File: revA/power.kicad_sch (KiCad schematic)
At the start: 58 parts, among them J9 Conn_02x02_Top_Bottom, Q1 MMBT4401WT1G, Q3 BSZ180, Q3 MMDT2222A, Q4 IRLML2803, Q6 MMDT2222A, Q9 MMDT2222A, U25 AP2161W, U3 MCP1700T-50, U4 MCP1700T-33, U5 MCP1700T-33, U6 ATL431BQ

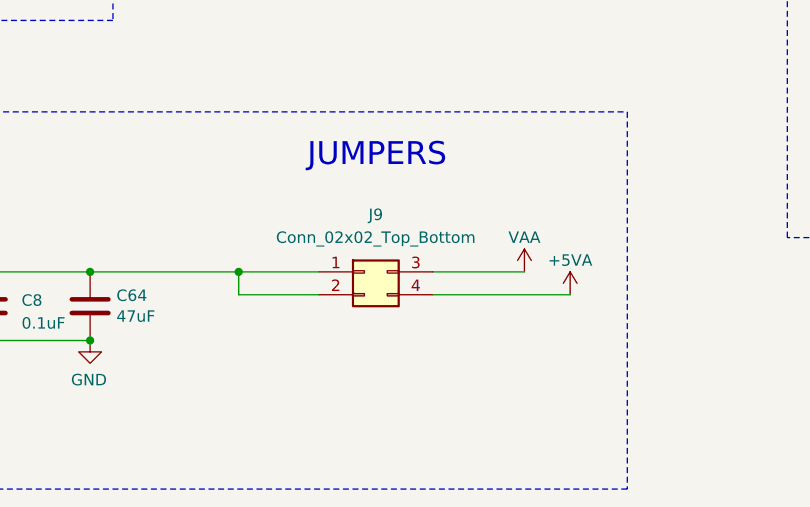
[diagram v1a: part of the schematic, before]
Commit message: placement
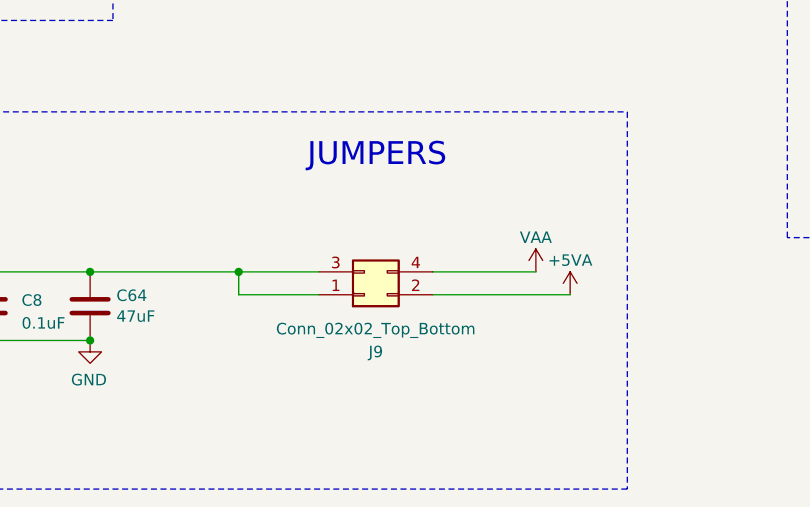
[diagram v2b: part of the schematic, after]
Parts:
- J9: symbol Connector_Generic:Conn_02x02_Top_Bottom -> Connector_Generic:Conn_02x02_Odd_Even
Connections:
- net +5VA: now also J9.2 (Pin_2); no longer J9.4 (Pin_4)
- net VAA: now also J9.4 (Pin_4); no longer J9.3 (Pin_3)
- net at C64.1, C8.1, J9.1 (Pin_1)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: now also J9.3 (Pin_3); no longer J9.2 (Pin_2)
- removed net +3V3: C13.1, C16.1, C17.1, R8.2, R87.1, R9.1, TP3.1, TP3.1, TP3.1, U4.3 (VO), U5.3 (VO), U6.2 (K)
- new net +1V65A: C17.1, R8.2, R9.1, TP3.1, U6.2 (K)
- new net +3V3A: C16.1, TP3.1, U5.3 (VO)
- new net +3V3D: C13.1, R87.1, TP3.1, U4.3 (VO)
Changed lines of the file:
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@@
     (stroke (width 0) (type default))
   )
-  (wire (pts (xy 182.88 215.9) (xy 193.04 215.9))
+  (wire (pts (xy 182.88 218.44) (xy 198.12 218.44))
     (stroke (width 0) (type default))
   )
@@
     (stroke (width 0) (type default))
   )
-  (wire (pts (xy 161.29 215.9) (xy 170.18 215.9))
-    (stroke (width 0) (type default))
-  )
   (wire (pts (xy 80.01 161.29) (xy 87.63 161.29))
     (stroke (width 0) (type default))
@@
     (stroke (width 0) (type default))
   )
+  (wire (pts (xy 161.29 215.9) (xy 170.18 215.9))
+    (stroke (width 0) (type default))
+  )
   (wire (pts (xy 63.5 55.88) (xy 95.25 55.88))
     (stroke (width 0) (type default))
@@
     (stroke (width 0) (type default))
   )
-  (wire (pts (xy 182.88 218.44) (xy 198.12 218.44))
+  (wire (pts (xy 182.88 215.9) (xy 194.31 215.9))
     (stroke (width 0) (type default))
   )
@@
       (effects (font (size 1.27 1.27)) hide)
     )
+    (property "Manufacturer" "" (at 351.79 170.18 0)
+      (effects (font (size 1.27 1.27)) hide)
+    )
+    (property "Mfr. Part No" "" (at 351.79 170.18 0)
+      (effects (font (size 1.27 1.27)) hide)
+    )
+    (property "Description" "" (at 351.79 170.18 0)
+      (effects (font (size 1.27 1.27)) hide)
+    )
     (pin "1")
     (instances
@@
       (effects (font (size 1.27 1.27)) hide)
     )
+    (property "Manufacturer" "" (at 309.88 175.26 0)
+      (effects (font (size 1.27 1.27)) hide)
+    )
+    (property "Mfr. Part No" "" (at 309.88 175.26 0)
+      (effects (font (size 1.27 1.27)) hide)
+    )
+    (property "Description" "" (at 309.88 175.26 0)
+      (effects (font (size 1.27 1.27)) hide)
+    )
     (pin "1")
     (instances
@@
     )
   )
-  (symbol (lib_id "Connector_Generic:Conn_02x02_Top_Bottom") (at 175.26 215.9 0) (unit 1)
+  (symbol (lib_id "Connector_Generic:Conn_02x02_Odd_Even") (at 175.26 218.44 0) (mirror x) (unit 1)
     (in_bom yes) (on_board yes) (dnp no)
-    (property "Reference" "J9" (at 176.53 209.55 0)
+    (property "Reference" "J9" (at 176.53 224.79 0)
       (effects (font (size 1.27 1.27)))
     )
-    (property "Value" "Conn_02x02_Top_Bottom" (at 176.53 212.09 0)
+    (property "Value" "Conn_02x02_Top_Bottom" (at 176.53 222.25 0)
       (effects (font (size 1.27 1.27)))
     )
-    (property "Footprint" "Connector_PinHeader_2.54mm:PinHeader_2x02_P2.54mm_Vertical_SMD" (at 175.26 215.9 0)
+    (property "Footprint" "Connector_PinHeader_2.54mm:PinHeader_2x02_P2.54mm_Vertical_SMD" (at 175.26 218.44 0)
+      (effects (font (size 1.27 1.27)) hide)
+    )
+    (property "Datasheet" "~" (at 175.26 218.44 0)
+      (effects (font (size 1.27 1.27)) hide)
+    )
+    (property "Manufacturer" "" (at 175.26 218.44 0)
       (effects (font (size 1.27 1.27)) hide)
     )
-    (property "Datasheet" "~" (at 175.26 215.9 0)
+    (property "Mfr. Part No" "" (at 175.26 218.44 0)
+      (effects (font (size 1.27 1.27)) hide)
+    )
+    (property "Description" "" (at 175.26 218.44 0)
       (effects (font (size 1.27 1.27)) hide)
     )
@@
       (effects (font (size 1.27 1.27)) hide)
     )
+    (property "Manufacturer" "" (at 309.88 160.02 0)
+      (effects (font (size 1.27 1.27)) hide)
+    )
+    (property "Mfr. Part No" "" (at 309.88 160.02 0)
+      (effects (font (size 1.27 1.27)) hide)
+    )
+    (property "Description" "" (at 309.88 160.02 0)
+      (effects (font (size 1.27 1.27)) hide)
+    )
     (pin "1")
     (instances
@@
       (effects (font (size 1.27 1.27)) hide)
     )
+    (property "Manufacturer" "" (at 281.94 184.15 0)
+      (effects (font (size 1.27 1.27)) hide)
+    )
+    (property "Mfr. Part No" "" (at 281.94 184.15 0)
+      (effects (font (size 1.27 1.27)) hide)
+    )
+    (property "Description" "" (at 281.94 184.15 0)
+      (effects (font (size 1.27 1.27)) hide)
+    )
     (pin "1")
     (instances
@@
       (effects (font (size 1.27 1.27)) hide)
     )
+    (property "Manufacturer" "" (at 271.78 45.72 0)
+      (effects (font (size 1.27 1.27)) hide)
+    )
+    (property "Mfr. Part No" "" (at 271.78 45.72 0)
+      (effects (font (size 1.27 1.27)) hide)
+    )
+    (property "Description" "" (at 271.78 45.72 0)
+      (effects (font (size 1.27 1.27)) hide)
+    )
     (pin "1")
     (instances
@@
       (effects (font (size 1.27 1.27)) hide)
     )
+    (property "Manufacturer" "" (at 309.88 182.88 0)
+      (effects (font (size 1.27 1.27)) hide)
+    )
+    (property "Mfr. Part No" "" (at 309.88 182.88 0)
+      (effects (font (size 1.27 1.27)) hide)
+    )
+    (property "Description" "" (at 309.88 182.88 0)
+      (effects (font (size 1.27 1.27)) hide)
+    )
     (pin "1")
     (instances
@@
       (effects (font (size 1.27 1.27)) hide)
     )
+    (property "Manufacturer" "" (at 271.78 137.16 0)
+      (effects (font (size 1.27 1.27)) hide)
+    )
+    (property "Mfr. Part No" "" (at 271.78 137.16 0)
+      (effects (font (size 1.27 1.27)) hide)
+    )
+    (property "Description" "" (at 271.78 137.16 0)
+      (effects (font (size 1.27 1.27)) hide)
+    )
     (pin "1")
     (instances
@@
     )
   )
-  (symbol (lib_id "power:VAA") (at 193.04 215.9 0) (unit 1)
+  (symbol (lib_id "power:VAA") (at 194.31 215.9 0) (unit 1)
     (in_bom yes) (on_board yes) (dnp no) (fields_autoplaced)
-    (property "Reference" "#PWR017" (at 193.04 219.71 0)
+    (property "Reference" "#PWR017" (at 194.31 219.71 0)
       (effects (font (size 1.27 1.27)) hide)
     )
-    (property "Value" "VAA" (at 193.04 212.09 0)
+    (property "Value" "VAA" (at 194.31 212.09 0)
       (effects (font (size 1.27 1.27)))
     )
-    (property "Footprint" "" (at 193.04 215.9 0)
+    (property "Footprint" "" (at 194.31 215.9 0)
       (effects (font (size 1.27 1.27)) hide)
     )
-    (property "Datasheet" "" (at 193.04 215.9 0)
+    (property "Datasheet" "" (at 194.31 215.9 0)
       (effects (font (size 1.27 1.27)) hide)
     )
